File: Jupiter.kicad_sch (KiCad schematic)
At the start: 347 parts, among them J1 Connector_USB_C_Receptacle_US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, SW1 SW_Push, U1 ATmega32U4-M, U2 PRTR5V0U2X, Y1 Crystal_GND24_Small

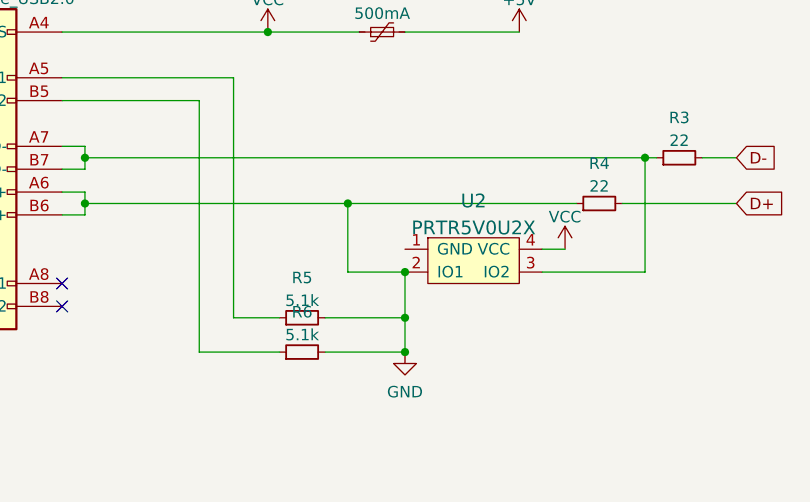
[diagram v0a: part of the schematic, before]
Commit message: Finished trace routing
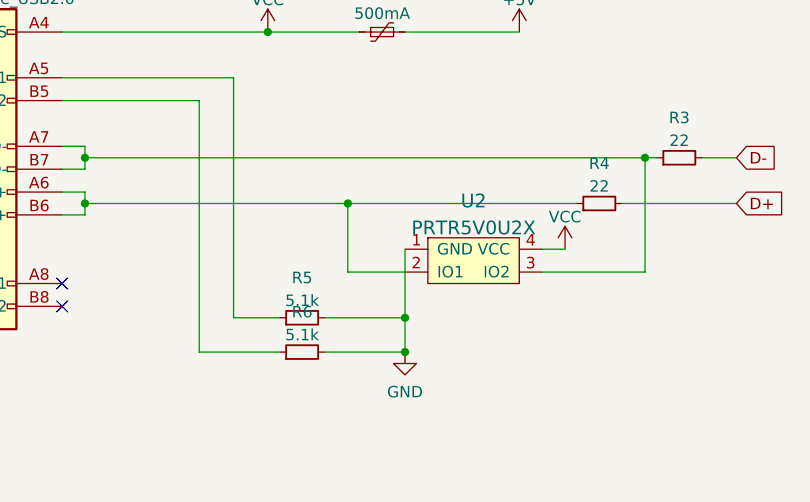
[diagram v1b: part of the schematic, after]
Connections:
- net GND: now also U2.1 (GND); no longer J1.A6 (D+), J1.B6 (D+), R4.1, U2.2 (IO1)
- new net: J1.A6 (D+), J1.B6 (D+), R4.1, U2.2 (IO1)
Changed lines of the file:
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@@
   (junction (at 332.74 265.43) (diameter 0) (color 0 0 0 0)
-  )
-  (junction (at 317.5 381) (diameter 0) (color 0 0 0 0)
   )
   (junction (at 472.44 242.57) (diameter 0) (color 0 0 0 0)
@@
     (stroke (width 0) (type default) (color 0 0 0 0))
   )
-  (wire (pts (xy 317.5 381) (xy 317.5 386.08))
-    (stroke (width 0) (type default) (color 0 0 0 0))
-  )
+  (wire (pts (xy 317.5 378.46) (xy 317.5 386.08))
+    (stroke (width 0) (type default) (color 0 0 0 0))
+  )
